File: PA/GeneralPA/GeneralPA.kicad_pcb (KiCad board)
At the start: 4 copper layers, 175 x 80.4 mm, 130 parts, among them J1 FAN, J2 RFin, J3 RFout, J4 FAN, J5 SWR, J6 48v_PAD, J7 48v_PAD, Q1 2N3904, Q2 IRF510, Q3 IRF510, Q4 2sc5706, Q5 2sc5706, Q6 BC548, T1 Transformer_1P_1S, T2 Transformer_1P_1S, T3 Transformer_T100, T4 Transformer_1P_1S, U1 LM317HVT, U2 LM7812_TO220

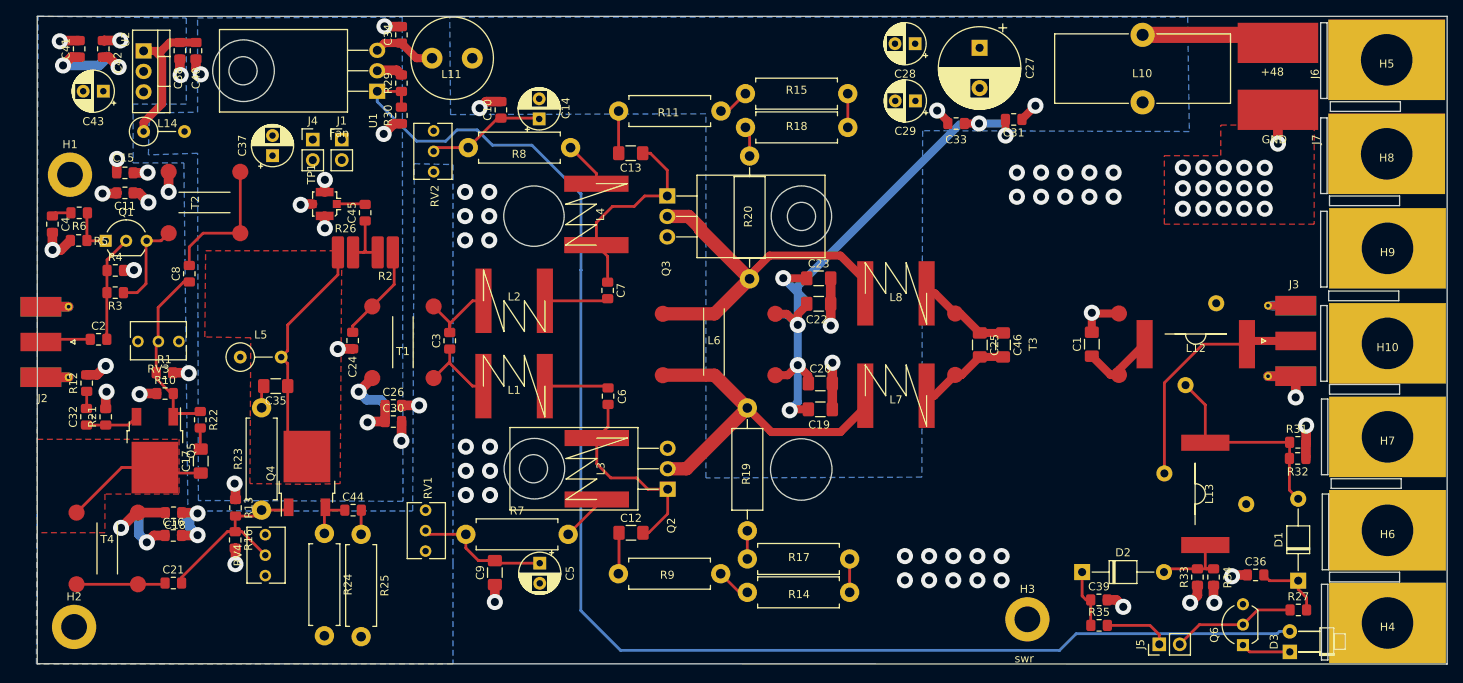
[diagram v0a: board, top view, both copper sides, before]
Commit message: add missed files
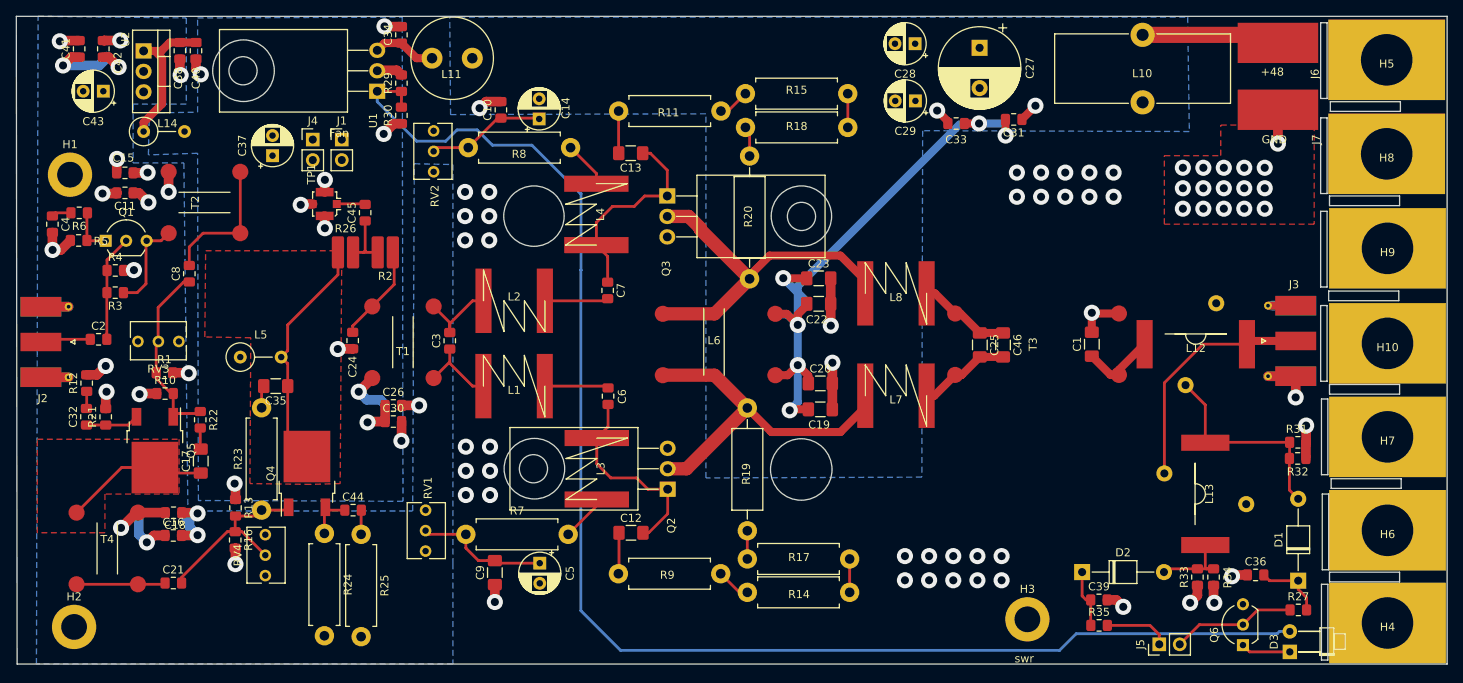
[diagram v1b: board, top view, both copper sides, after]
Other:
- board size 175 x 80.4 mm -> 177.6 x 80.4 mm
